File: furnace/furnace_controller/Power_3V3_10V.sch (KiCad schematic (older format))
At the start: 28 parts

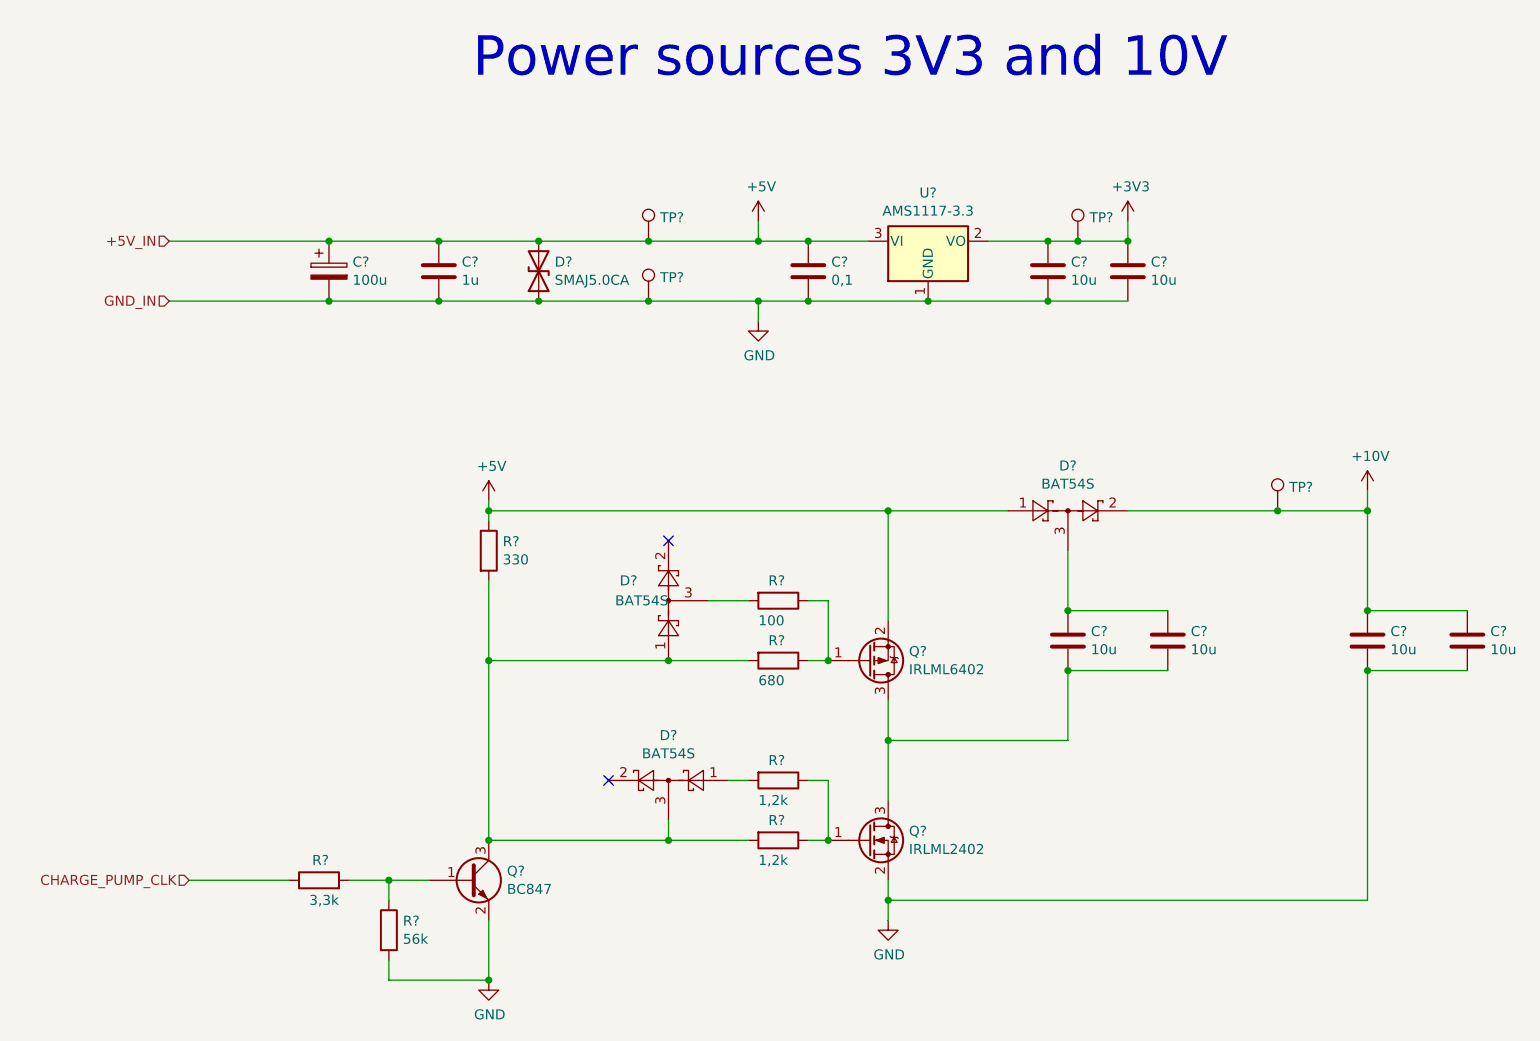
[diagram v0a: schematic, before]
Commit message: Add files via upload
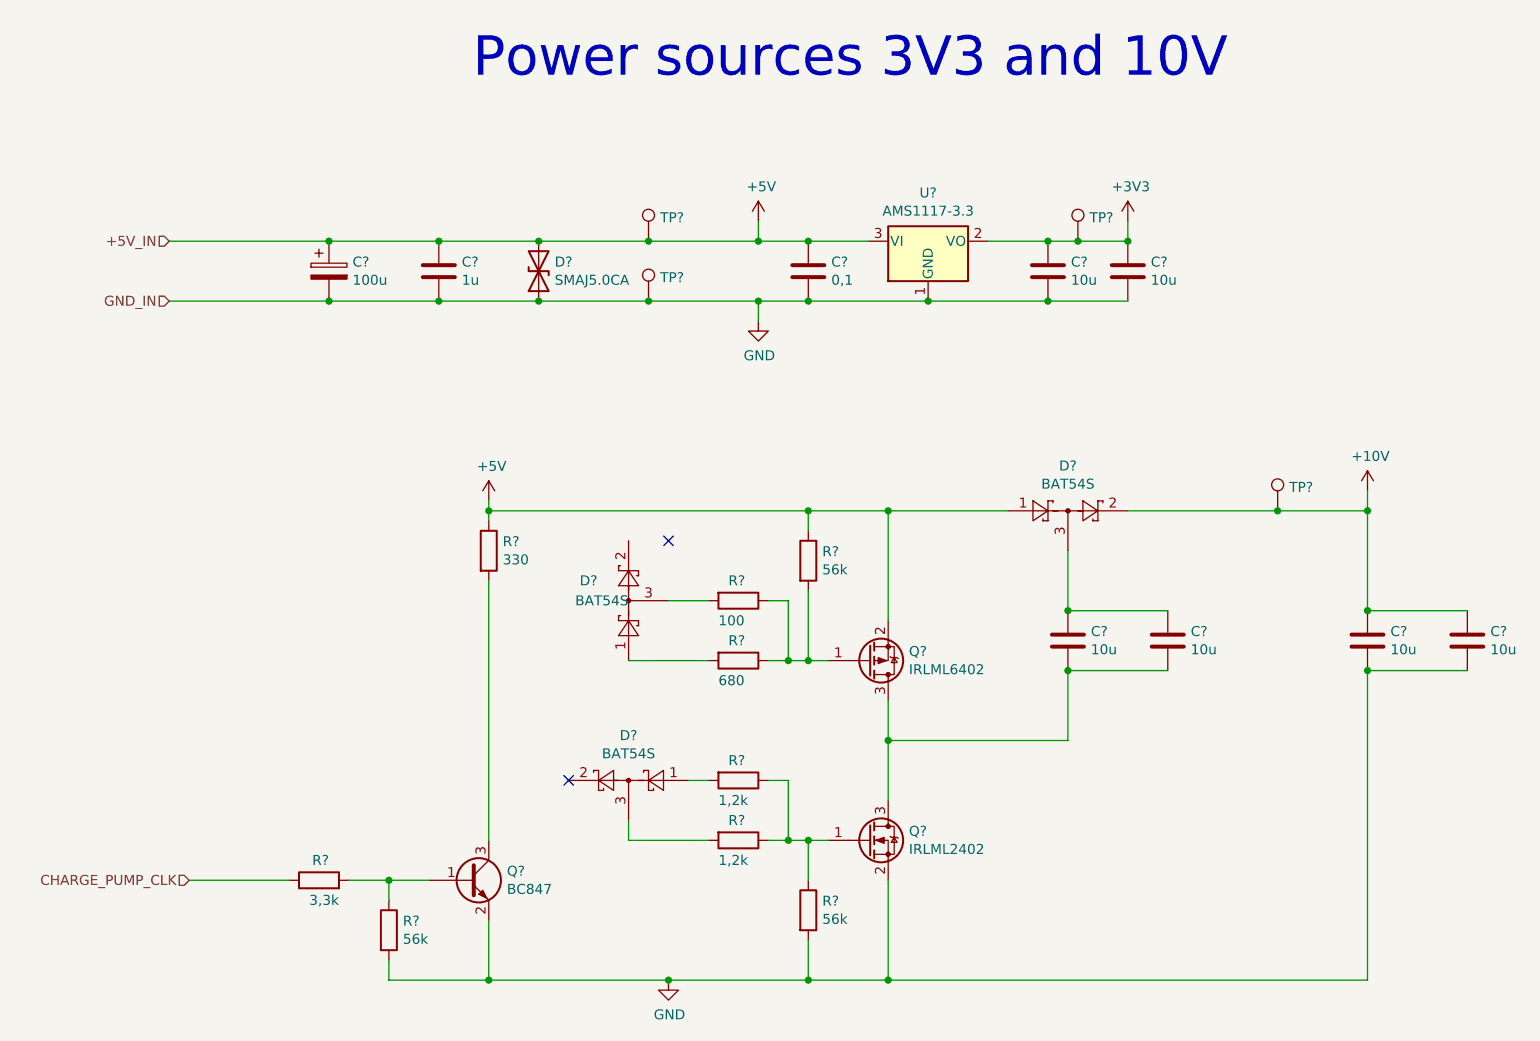
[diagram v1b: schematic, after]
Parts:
- added R? (x2): 56k, Resistor_SMD:R_0603_1608Metric_Pad0.98x0.95mm_HandSolder, symbol Device:R
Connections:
- net +5V: now also R?.1
- net GND: now also R?.2
- net at Q?.1 (G), R?.1, R?.1: now also R?.2
- net at Q?.1 (G), R?.1, R?.1: now also R?.1
- new net: D?.1, R?.2
- new net: D?.3, R?.2
- new net: Q?.3 (C), R?.2
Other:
- moved on the sheet: D?, R?
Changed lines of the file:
@@
 L Diode:BAT54S D?
 U 1 1 60A281E0
-P 5400 4350
-F 0 "D?" V 5500 4550 50  0000 C CNN
-F 1 "BAT54S" V 5400 4484 50  0000 C CNN
-F 2 "Package_TO_SOT_SMD:SOT-23" H 5475 4475 50  0001 L CNN
-F 3 "https://www.diodes.com/assets/Datasheets/ds11005.pdf" H 5280 4350 50  0001 C CNN
-	1    5400 4350
+P 5200 4350
+F 0 "D?" V 5300 4550 50  0000 C CNN
+F 1 "BAT54S" V 5200 4484 50  0000 C CNN
+F 2 "Package_TO_SOT_SMD:SOT-23" H 5275 4475 50  0001 L CNN
+F 3 "https://www.diodes.com/assets/Datasheets/ds11005.pdf" H 5080 4350 50  0001 C CNN
+	1    5200 4350
 	0    -1   -1   0
 $EndComp
@@
 L Diode:BAT54S D?
 U 1 1 60A2A42D
-P 5400 5250
-F 0 "D?" H 5400 5475 50  0000 C CNN
-F 1 "BAT54S" H 5400 5384 50  0000 C CNN
-F 2 "Package_TO_SOT_SMD:SOT-23" H 5475 5375 50  0001 L CNN
-F 3 "https://www.diodes.com/assets/Datasheets/ds11005.pdf" H 5280 5250 50  0001 C CNN
-	1    5400 5250
+P 5200 5250
+F 0 "D?" H 5200 5475 50  0000 C CNN
+F 1 "BAT54S" H 5200 5384 50  0000 C CNN
+F 2 "Package_TO_SOT_SMD:SOT-23" H 5275 5375 50  0001 L CNN
+F 3 "https://www.diodes.com/assets/Datasheets/ds11005.pdf" H 5080 5250 50  0001 C CNN
+	1    5200 5250
 	-1   0    0    -1
 $EndComp
@@
 L Device:R R?
 U 1 1 60A272DA
-P 5950 4350
+P 5750 4350
 AR Path="/60A272DA" Ref="R?"  Part="1"
 AR Path="/609FED99/60A272DA" Ref="R?"  Part="1"
-F 0 "R?" V 5850 4300 50  0000 L CNN
-F 1 "100" V 6050 4250 50  0000 L CNN
-F 2 "Resistor_SMD:R_0603_1608Metric_Pad0.98x0.95mm_HandSolder" V 5880 4350 50  0001 C CNN
-F 3 "~" H 5950 4350 50  0001 C CNN
-	1    5950 4350
+F 0 "R?" V 5650 4300 50  0000 L CNN
+F 1 "100" V 5850 4250 50  0000 L CNN
+F 2 "Resistor_SMD:R_0603_1608Metric_Pad0.98x0.95mm_HandSolder" V 5680 4350 50  0001 C CNN
+F 3 "~" H 5750 4350 50  0001 C CNN
+	1    5750 4350
 	0    1    1    0
 $EndComp
@@
 L Device:R R?
 U 1 1 60A440E9
-P 5950 4650
+P 5750 4650
 AR Path="/60A440E9" Ref="R?"  Part="1"
 AR Path="/609FED99/60A440E9" Ref="R?"  Part="1"
-F 0 "R?" V 5850 4600 50  0000 L CNN
-F 1 "680" V 6050 4550 50  0000 L CNN
-F 2 "Resistor_SMD:R_0603_1608Metric_Pad0.98x0.95mm_HandSolder" V 5880 4650 50  0001 C CNN
-F 3 "~" H 5950 4650 50  0001 C CNN
-	1    5950 4650
+F 0 "R?" V 5650 4600 50  0000 L CNN
+F 1 "680" V 5850 4550 50  0000 L CNN
+F 2 "Resistor_SMD:R_0603_1608Metric_Pad0.98x0.95mm_HandSolder" V 5680 4650 50  0001 C CNN
+F 3 "~" H 5750 4650 50  0001 C CNN
+	1    5750 4650
 	0    1    1    0
 $EndComp
@@
 L Device:R R?
 U 1 1 60A443B1
-P 5950 5250
+P 5750 5250
 AR Path="/60A443B1" Ref="R?"  Part="1"
 AR Path="/609FED99/60A443B1" Ref="R?"  Part="1"
-F 0 "R?" V 5850 5200 50  0000 L CNN
-F 1 "1,2k" V 6050 5150 50  0000 L CNN
-F 2 "Resistor_SMD:R_0603_1608Metric_Pad0.98x0.95mm_HandSolder" V 5880 5250 50  0001 C CNN
-F 3 "~" H 5950 5250 50  0001 C CNN
-	1    5950 5250
+F 0 "R?" V 5650 5200 50  0000 L CNN
+F 1 "1,2k" V 5850 5150 50  0000 L CNN
+F 2 "Resistor_SMD:R_0603_1608Metric_Pad0.98x0.95mm_HandSolder" V 5680 5250 50  0001 C CNN
+F 3 "~" H 5750 5250 50  0001 C CNN
+	1    5750 5250
 	0    1    1    0
 $EndComp
@@
 L Device:R R?
 U 1 1 60A44627
-P 5950 5550
+P 5750 5550
 AR Path="/60A44627" Ref="R?"  Part="1"
 AR Path="/609FED99/60A44627" Ref="R?"  Part="1"
-F 0 "R?" V 5850 5500 50  0000 L CNN
-F 1 "1,2k" V 6050 5450 50  0000 L CNN
-F 2 "Resistor_SMD:R_0603_1608Metric_Pad0.98x0.95mm_HandSolder" V 5880 5550 50  0001 C CNN
-F 3 "~" H 5950 5550 50  0001 C CNN
-	1    5950 5550
+F 0 "R?" V 5650 5500 50  0000 L CNN
+F 1 "1,2k" V 5850 5450 50  0000 L CNN
+F 2 "Resistor_SMD:R_0603_1608Metric_Pad0.98x0.95mm_HandSolder" V 5680 5550 50  0001 C CNN
+F 3 "~" H 5750 5550 50  0001 C CNN
+	1    5750 5550
 	0    1    1    0
 $EndComp
@@
 	4500 3850 4500 3900
 Wire Wire Line
-	5800 5550 5400 5550
-Wire Wire Line
-	5400 5450 5400 5550
-Connection ~ 5400 5550
-Wire Wire Line
-	5400 5550 4500 5550
-Wire Wire Line
-	6100 4350 6200 4350
-Wire Wire Line
-	6200 4350 6200 4650
-Wire Wire Line
-	6200 4650 6100 4650
-Connection ~ 6200 4650
-Wire Wire Line
-	5700 5250 5800 5250
-Wire Wire Line
-	6100 5250 6200 5250
-Wire Wire Line
-	6200 5250 6200 5550
-Wire Wire Line
-	6200 5550 6100 5550
-Connection ~ 6200 5550
+	5600 5550 5200 5550
+Wire Wire Line
+	5200 5450 5200 5550
+Wire Wire Line
+	5500 5250 5600 5250
 Wire Wire Line
 	6500 4850 6500 5050
@@
 Wire Wire Line
 	4500 3900 4500 3950
-NoConn ~ 5100 5250
+NoConn ~ 4900 5250
 Text HLabel 3000 5750 0    50   Input ~ 0
 CHARGE_PUMP_CLK
@@
 Connection ~ 8900 3900
 Connection ~ 8900 4400
-Wire Wire Line
-	8900 4700 8900 5850
-Wire Wire Line
-	8900 5850 6500 5850
-Wire Wire Line
-	6500 5850 6500 5750
 Connection ~ 8900 4700
-Wire Wire Line
-	6500 5850 6500 5950
-Connection ~ 6500 5850
-$Comp
-L power:GND #PWR?
-U 1 1 60AB9561
-P 6500 5950
-F 0 "#PWR?" H 6500 5700 50  0001 C CNN
-F 1 "GND" H 6505 5777 50  0000 C CNN
-F 2 "" H 6500 5950 50  0001 C CNN
-F 3 "" H 6500 5950 50  0001 C CNN
-	1    6500 5950
-	1    0    0    -1
-$EndComp
 $Comp
 L Connector:TestPoint TP?
@@
 $EndComp
 Wire Wire Line
-	4500 4650 5400 4650
-Connection ~ 4500 4650
-Wire Wire Line
-	4500 4250 4500 4650
-Wire Wire Line
-	4500 3900 6500 3900
-Wire Wire Line
-	5400 4650 5800 4650
+	5200 4650 5600 4650
 Wire Wire Line
 	6500 5050 6500 5350
-Connection ~ 5400 4650
-Wire Wire Line
-	5600 4350 5800 4350
+Wire Wire Line
+	5400 4350 5600 4350
 NoConn ~ 5400 4050
 Wire Wire Line
@@
 Text HLabel 2900 2850 0    50   Input ~ 0
 GND_IN
-Wire Wire Line
-	4500 4650 4500 5550
 $Comp
 L Transistor_BJT:BC847 Q?
@@
 AR Path="/609C9D41/60B184A0" Ref="Q?"  Part="1"
 AR Path="/60B39FE1/60B184A0" Ref="Q?"  Part="1"
+AR Path="/609FED99/60B184A0" Ref="Q?"  Part="1"
 F 0 "Q?" H 4591 5796 50  0000 L CNN
 F 1 "BC847" H 4591 5705 50  0000 L CNN
@@
 AR Path="/60B184A6" Ref="R?"  Part="1"
 AR Path="/60B39FE1/60B184A6" Ref="R?"  Part="1"
+AR Path="/609FED99/60B184A6" Ref="R?"  Part="1"
 F 0 "R?" H 4070 6046 50  0000 L CNN
 F 1 "56k" H 4070 5955 50  0000 L CNN
@@
 AR Path="/60B184AC" Ref="R?"  Part="1"
 AR Path="/60B39FE1/60B184AC" Ref="R?"  Part="1"
+AR Path="/609FED99/60B184AC" Ref="R?"  Part="1"
 F 0 "R?" V 3750 5700 50  0000 L CNN
 F 1 "3,3k" V 3550 5650 50  0000 L CNN
@@
 Wire Wire Line
 	4000 6150 4000 6250
-Connection ~ 4500 5550
 $Comp
 L power:GND #PWR?
 U 1 1 60B1D9CB
-P 4500 6250
-F 0 "#PWR?" H 4500 6000 50  0001 C CNN
-F 1 "GND" H 4505 6077 50  0000 C CNN
-F 2 "" H 4500 6250 50  0001 C CNN
-F 3 "" H 4500 6250 50  0001 C CNN
-	1    4500 6250
+P 5400 6250
+F 0 "#PWR?" H 5400 6000 50  0001 C CNN
+F 1 "GND" H 5405 6077 50  0000 C CNN
+F 2 "" H 5400 6250 50  0001 C CNN
+F 3 "" H 5400 6250 50  0001 C CNN
+	1    5400 6250
 	1    0    0    -1
 $EndComp
@@
 	4500 5950 4500 6250
 Connection ~ 4500 6250
+$Comp
+L Device:R R?
+U 1 1 60B13DFF
+P 6100 5900
+AR Path="/60B13DFF" Ref="R?"  Part="1"
+AR Path="/60B39FE1/60B13DFF" Ref="R?"  Part="1"
+AR Path="/609FED99/60B13DFF" Ref="R?"  Part="1"
+F 0 "R?" H 6170 5946 50  0000 L CNN
+F 1 "56k" H 6170 5855 50  0000 L CNN
+F 2 "Resistor_SMD:R_0603_1608Metric_Pad0.98x0.95mm_HandSolder" V 6030 5900 50  0001 C CNN
+F 3 "~" H 6100 5900 50  0001 C CNN
+	1    6100 5900
+	1    0    0    -1
+$EndComp
+Wire Wire Line
+	4500 4250 4500 5550
+$Comp
+L Device:R R?
+U 1 1 60B1B4E2
+P 6100 4150
+AR Path="/60B1B4E2" Ref="R?"  Part="1"
+AR Path="/60B39FE1/60B1B4E2" Ref="R?"  Part="1"
+AR Path="/609FED99/60B1B4E2" Ref="R?"  Part="1"
+F 0 "R?" H 6170 4196 50  0000 L CNN
+F 1 "56k" H 6170 4105 50  0000 L CNN
+F 2 "Resistor_SMD:R_0603_1608Metric_Pad0.98x0.95mm_HandSolder" V 6030 4150 50  0001 C CNN
+F 3 "~" H 6100 4150 50  0001 C CNN
+	1    6100 4150
+	1    0    0    -1
+$EndComp
+Wire Wire Line
+	4500 3900 6100 3900
+Wire Wire Line
+	6100 4000 6100 3900
+Connection ~ 6100 3900
+Wire Wire Line
+	6100 3900 6500 3900
+Wire Wire Line
+	5900 4650 6000 4650
+Connection ~ 6100 4650
+Wire Wire Line
+	6100 4650 6200 4650
+Wire Wire Line
+	4500 6250 5400 6250
+Wire Wire Line
+	8900 4700 8900 6250
+Wire Wire Line
+	5900 5550 6000 5550
+Wire Wire Line
+	6100 5750 6100 5550
+Connection ~ 6100 5550
+Wire Wire Line
+	6100 5550 6200 5550
+Wire Wire Line
+	6100 6050 6100 6250
+Connection ~ 6100 6250
+Wire Wire Line
+	6100 6250 6500 6250
+Wire Wire Line
+	5900 5250 6000 5250
+Wire Wire Line
+	6000 5250 6000 5550
+Connection ~ 6000 5550
+Wire Wire Line
+	6000 5550 6100 5550
+Wire Wire Line
+	6100 4300 6100 4650
+Wire Wire Line
+	5900 4350 6000 4350
+Wire Wire Line
+	6000 4350 6000 4650
+Connection ~ 6000 4650
+Wire Wire Line
+	6000 4650 6100 4650
+Connection ~ 5400 6250
+Wire Wire Line
+	5400 6250 6100 6250
+Wire Wire Line
+	6500 5750 6500 6250
+Connection ~ 6500 6250
+Wire Wire Line
+	6500 6250 8900 6250
 $EndSCHEMATC
